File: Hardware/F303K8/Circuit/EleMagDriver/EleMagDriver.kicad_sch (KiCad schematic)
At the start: 4 parts, among them IC1 TBD62083APG, IC2 TBD62083APG, J1 Conn_01x02_Female, U1 NUCLEO-F303K8

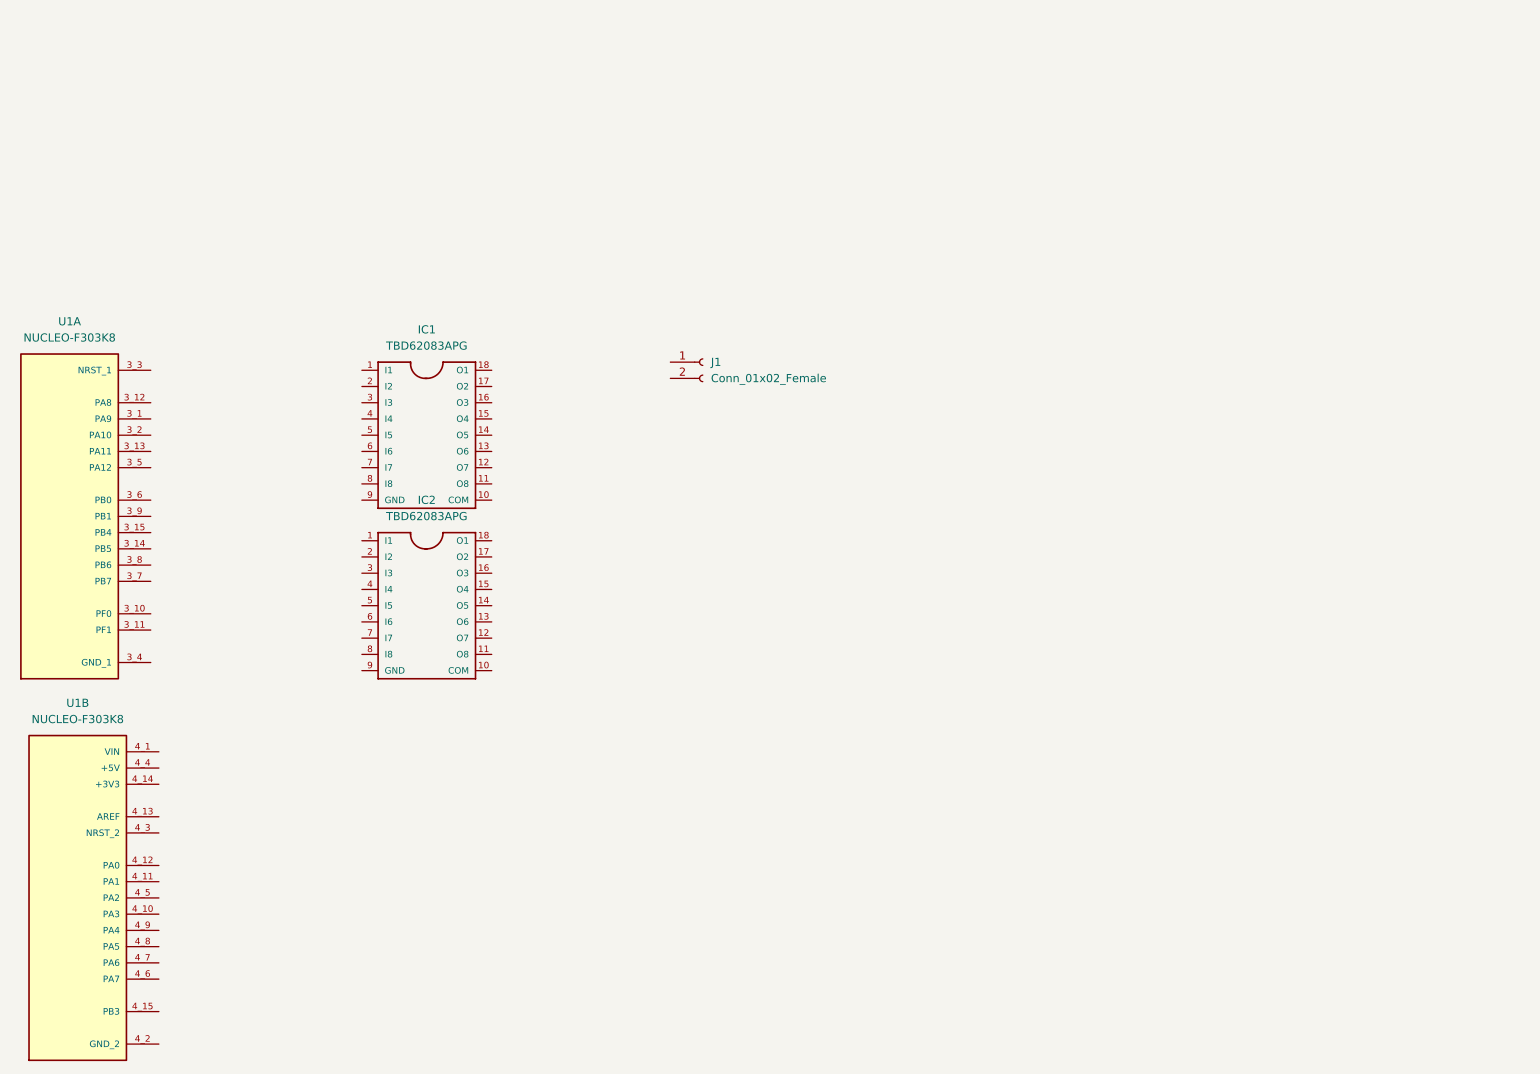
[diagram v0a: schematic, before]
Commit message: edit circuit
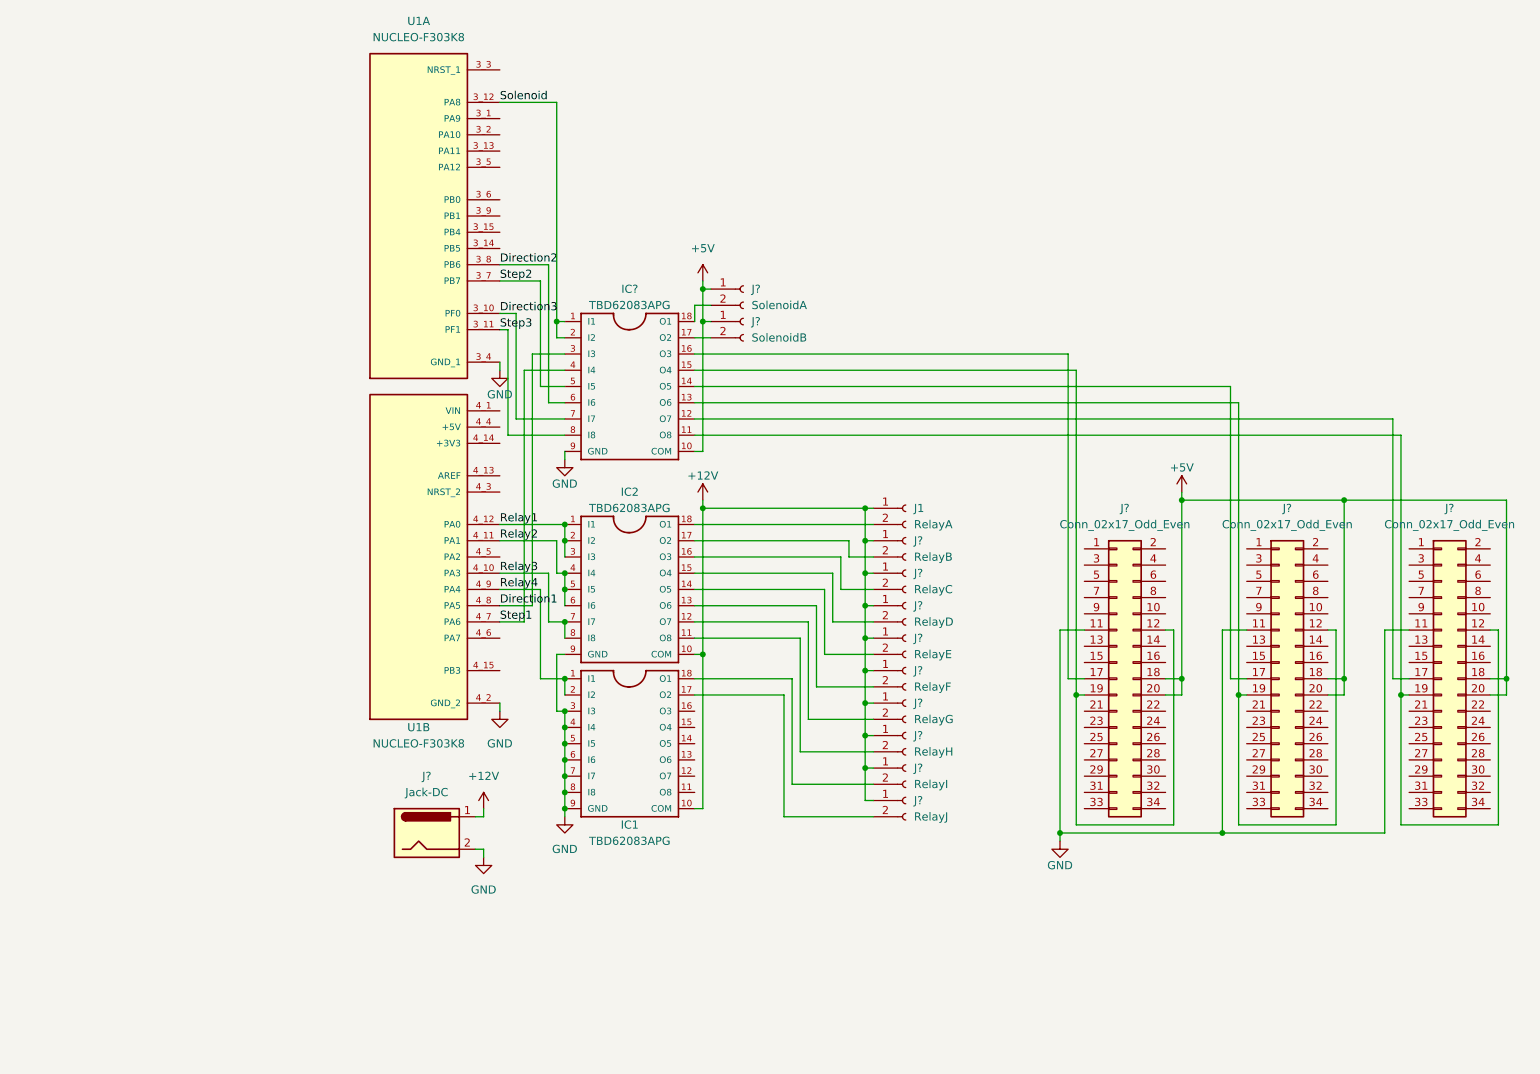
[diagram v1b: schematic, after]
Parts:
- added IC?: TBD62083APG, symbol TBD62083APG:TBD62083APG
- added J?: SolenoidA, symbol Connector:Conn_01x02_Female
- added J?: RelayD, symbol Connector:Conn_01x02_Female
- added J?: SolenoidB, symbol Connector:Conn_01x02_Female
- added J?: RelayB, symbol Connector:Conn_01x02_Female
- added J?: RelayH, symbol Connector:Conn_01x02_Female
- added J?: RelayE, symbol Connector:Conn_01x02_Female
- added J?: RelayJ, symbol Connector:Conn_01x02_Female
- added J?: RelayI, symbol Connector:Conn_01x02_Female
- added J? (x3): Conn_02x17_Odd_Even, symbol Connector_Generic:Conn_02x17_Odd_Even
- added J?: RelayF, symbol Connector:Conn_01x02_Female
- added J?: RelayG, symbol Connector:Conn_01x02_Female
- added J?: RelayC, symbol Connector:Conn_01x02_Female
- added J?: Jack-DC, symbol Connector:Jack-DC
- J1: value Conn_01x02_Female -> RelayA
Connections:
- net +12V: now reaches J1.1 (Pin_1)
- net +12V: now also IC1.10 (COM), IC2.10 (COM), J?.1, J?.1 (Pin_1), J?.1 (Pin_1), J?.1 (Pin_1), J?.1 (Pin_1), J?.1 (Pin_1), J?.1 (Pin_1), J?.1 (Pin_1), J?.1 (Pin_1), J?.1 (Pin_1)
- net at J1.2 (Pin_2): now also IC2.18 (O1)
- net Relay3: now reaches U1.4_10 (PA3)
- net Relay3: now also IC2.7 (I7), IC2.8 (I8)
- net Relay2: now reaches U1.4_11 (PA1)
- net Relay2: now also IC2.4 (I4), IC2.5 (I5), IC2.6 (I6)
- net Relay1: now reaches U1.4_12 (PA0)
- net Relay1: now also IC2.1 (I1), IC2.2 (I2), IC2.3 (I3)
- net GND: now reaches U1.4_2 (GND_2)
- net GND: now also IC1.3 (I3), IC1.4 (I4), IC1.5 (I5), IC1.6 (I6), IC1.7 (I7), IC1.8 (I8), IC1.9 (GND), IC2.9 (GND), U1.3_4 (GND_1), IC?.9 (GND), J?.11 (Pin_11), J?.11 (Pin_11), J?.11 (Pin_11), J?.2
- net Step1: now reaches U1.4_7 (PA6)
- net Step1: now also IC?.4 (I4)
- net Direction1: now reaches U1.4_8 (PA5)
- net Direction1: now also IC?.3 (I3)
- net Relay4: now reaches U1.4_9 (PA4)
- net Relay4: now also IC1.1 (I1), IC1.2 (I2)
- net Direction3: now reaches U1.3_10 (PF0)
- net Direction3: now also IC?.7 (I7)
- net Step3: now reaches U1.3_11 (PF1)
- net Step3: now also IC?.8 (I8)
- net Solenoid: now reaches U1.3_12 (PA8)
- net Solenoid: now also IC?.1 (I1), IC?.2 (I2)
- net Step2: now reaches U1.3_7 (PB7)
- net Step2: now also IC?.5 (I5)
- net Direction2: now reaches U1.3_8 (PB6)
- net Direction2: now also IC?.6 (I6)
- net at IC1.17 (O2): now also J?.2 (Pin_2)
- net at IC1.18 (O1): now also J?.2 (Pin_2)
- net at IC2.11 (O8): now also J?.2 (Pin_2)
- net at IC2.12 (O7): now also J?.2 (Pin_2)
- net at IC2.13 (O6): now also J?.2 (Pin_2)
- net at IC2.14 (O5): now also J?.2 (Pin_2)
- net at IC2.15 (O4): now also J?.2 (Pin_2)
- net at IC2.16 (O3): now also J?.2 (Pin_2)
- net at IC2.17 (O2): now also J?.2 (Pin_2)
- new net: IC?.18 (O1), J?.2 (Pin_2)
- new net: IC?.17 (O2), J?.2 (Pin_2)
- new net: IC?.11 (O8), J?.12 (Pin_12), J?.19 (Pin_19)
- new net: IC?.12 (O7), J?.17 (Pin_17)
- new net: IC?.13 (O6), J?.12 (Pin_12), J?.19 (Pin_19)
- new net: IC?.14 (O5), J?.17 (Pin_17)
- new net: IC?.15 (O4), J?.12 (Pin_12), J?.19 (Pin_19)
- new net: IC?.16 (O3), J?.17 (Pin_17)
- new net +5V: IC?.10 (COM), J?.1 (Pin_1), J?.1 (Pin_1), J?.18 (Pin_18), J?.18 (Pin_18), J?.18 (Pin_18), J?.20 (Pin_20), J?.20 (Pin_20), J?.20 (Pin_20)
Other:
- moved on the sheet: IC1, IC2, J1, U1A, U1B
